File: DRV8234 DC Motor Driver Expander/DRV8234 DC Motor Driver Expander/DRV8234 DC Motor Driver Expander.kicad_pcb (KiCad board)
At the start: 4 copper layers, 73.2 x 31.2 mm, 44 parts, among them IC1 DRV8234RTER, J1 POWER, J2 CNTRL_IN, J3 CNTRL_OUT, J4 I2C, J5 MOTOR

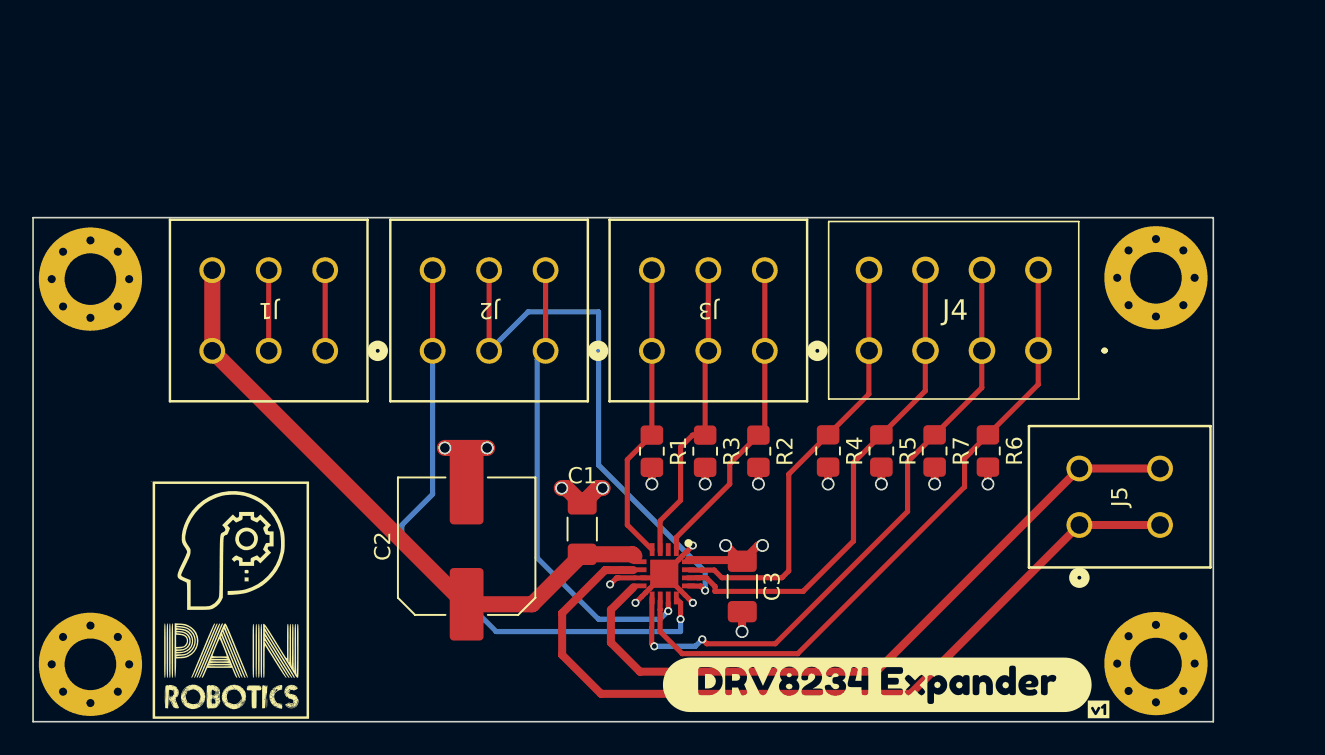
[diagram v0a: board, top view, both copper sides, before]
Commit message: V2
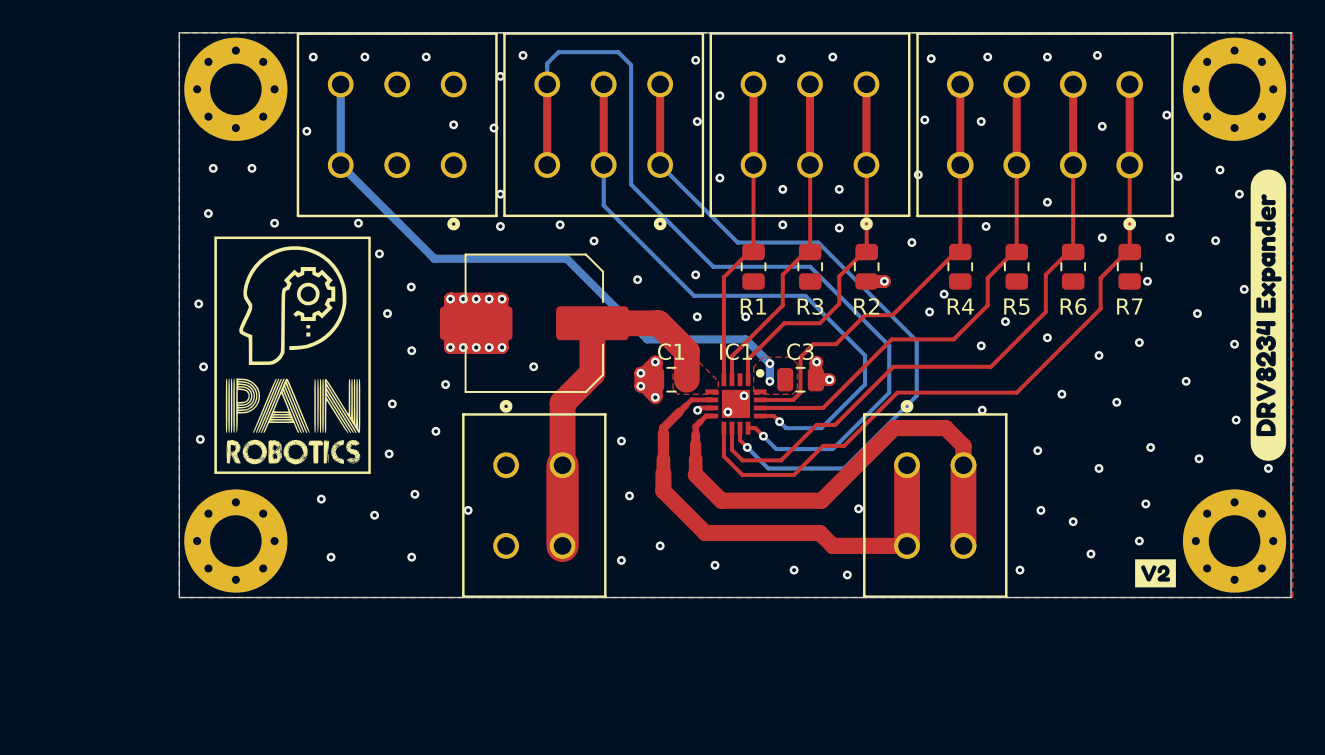
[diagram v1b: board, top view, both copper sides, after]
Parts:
- removed kibuzzard-65A6FC4F: G***, kibuzzard-65A6FC4F
- removed kibuzzard-65A7000E: G***, kibuzzard-65A7000E
- removed kibuzzard-65A7036D: G***, kibuzzard-65A7036D
- removed kibuzzard-65A7039D: G***, kibuzzard-65A7039D
- added J6: CONN_1862055, PCB Footprints:1862055, F.Cu at (110.0, 68.2)
- added kibuzzard-66A118A5: G***, kibuzzard-66A118A5, B.Cu at (113.5, 70.7)
- added kibuzzard-66A118C9: G***, kibuzzard-66A118C9, B.Cu at (122.0, 94.3)
- added kibuzzard-66A1197F: G***, kibuzzard-66A1197F, B.Cu at (120.2, 89.2)
- added kibuzzard-66A11A0B: G***, kibuzzard-66A11A0B, B.Cu at (117.0, 76.0)
- added kibuzzard-66A11A2A: G***, kibuzzard-66A11A2A, B.Cu at (110.0, 75.8)
- added kibuzzard-66A11B65: G***, kibuzzard-66A11B65, F.Cu at (167.5, 82.5)
- added kibuzzard-66A13964: G***, kibuzzard-66A13964, F.Cu at (160.5, 98.5)
- C1, C3: footprint Capacitor_SMD:C_1206_3216Metric_Pad1.33x1.80mm_HandSolder -> Capacitor_SMD:C_0805_2012Metric
- IC1: footprint DRV8234 Footprint:QFN50P300X300X80-17N-D -> PCB Footprints:DRV8234RTER
- J1: value POWER -> CONN_1862042; footprint 1862055 Footprint:CONN_1862055 -> PCB Footprints:1862042
- J2: value CNTRL_IN -> CONN_1862055; footprint 1862055 Footprint:CONN_1862055 -> PCB Footprints:1862055
- J3: value CNTRL_OUT -> CONN_1862055; footprint 1862055 Footprint:CONN_1862055 -> PCB Footprints:1862055
- J4: value I2C -> 1862068; footprint 1862068 Footprint:1862068 -> PCB Footprints:1862068
- J5: value MOTOR -> CONN_1862042; footprint 1862042 Footprint:CONN_1862042 -> PCB Footprints:1862042
- R1, R3: value 10K -> 10k; footprint Resistor_SMD:R_0805_2012Metric_Pad1.20x1.40mm_HandSolder -> Resistor_SMD:R_0805_2012Metric
- R2: value 8.45K -> 1.2k; footprint Resistor_SMD:R_0805_2012Metric_Pad1.20x1.40mm_HandSolder -> Resistor_SMD:R_0805_2012Metric
- R4, R5, R6, R7: value 2.2K -> 2.2k; footprint Resistor_SMD:R_0805_2012Metric_Pad1.20x1.40mm_HandSolder -> Resistor_SMD:R_0805_2012Metric
- moved J1 27.6 mm to (123.8, 96.8), turned to 0 degrees
- moved kibuzzard-65A6FC26 21.8 mm to (123.8, 88.2), turned to 90 degrees
- moved R7 16.6 mm to (158.9, 79.5), turned to 90 degrees
- moved G*** 15.7 mm to (107.0, 85.0)
- moved H1 14.8 mm to (103.5, 68.5)
- moved C2 14.4 mm to (122.0, 83.0), turned to 180 degrees
- moved R5 14.2 mm to (151.9, 79.5), turned to 90 degrees
- moved R4 14.1 mm to (148.4, 79.5), turned to 90 degrees
- moved kibuzzard-65A6FC0C 14.0 mm to (113.5, 75.7)
- moved kibuzzard-65A6FFF9 13.5 mm to (126.3, 70.7), turned to 0 degrees
- moved J2 13.5 mm to (122.8, 68.2)
- moved kibuzzard-65A6FCD9 13.5 mm to (122.8, 75.5)
- moved kibuzzard-65A6FCAC 13.5 mm to (126.3, 75.4)
- moved kibuzzard-65A6FCCE 13.5 mm to (129.8, 76.5), turned to -90 degrees
- moved C3 13.3 mm to (138.5, 86.5), turned to 0 degrees
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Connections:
- C1 pad 1: VCC -> VM
- C2 pad 1: VCC -> VM
- C3 pad 1: +5V -> +3V3
- IC1 pad 16: +5V -> +3V3
- IC1 pad 5: VCC -> VM
- J1 pad 1: +5V -> GND
- J1 pad 2: +5V -> GND
- J1 pad 3: GND -> VM
- J1 pad 4: GND -> VM
- J4 pad 1: A0 -> A1
- J4 pad 2: A0 -> A1
- J4 pad 3: A1 -> A0
- J4 pad 4: A1 -> A0
- R1 pad 1: NFAULT -> VCC_MCU
- R1 pad 2: +5V -> NFAULT
- R3 pad 1: RC_OUT -> VCC_MCU
- R3 pad 2: +5V -> RC_OUT
- R4 pad 1: SCL -> VCC_MCU
- R4 pad 2: +5V -> SCL
- R5 pad 1: SDA -> VCC_MCU
- R5 pad 2: +5V -> SDA
- R6 pad 1: A0 -> VCC_MCU
- R6 pad 2: +5V -> A0
- R7 pad 1: A1 -> VCC_MCU
- R7 pad 2: +5V -> A1
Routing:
- net VCC: track 39.0 -> 0.00 mm
- net +3V3: track 0.00 -> 37.8 mm, vias 0 -> 2
- net GND: track 15.7 -> 42.1 mm, vias 10 -> 96
- net VM: track 0.00 -> 22.9 mm
- net OUT1: track 50.4 -> 29.1 mm
- net +5V: track 17.7 -> 0.00 mm, vias 8 -> 0
- net NSLEEP: track 28.5 -> 43.1 mm
- net IN2: track 38.8 -> 53.3 mm
- net OUT2: track 44.0 -> 30.1 mm
- net A1: track 39.5 -> 44.6 mm, vias 2 -> 0
- net (no net): track 4.67 -> 0.00 mm
- net IN1: track 33.9 -> 37.3 mm
- net IPROPI: track 19.6 -> 22.8 mm
- net RC_OUT: track 19.1 -> 20.5 mm
- net A0: track 41.1 -> 39.9 mm
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- added copper zone on F.Cu, net +3V3
- added copper zone on In2.Cu, net GND
- added copper zone on B.Cu, net VCC_MCU
- added copper zone on F.Cu, net VCC_MCU
- added copper zone on F.Cu, net VM
- removed copper zone on In2.Cu, net +5V
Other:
- board size 73.2 x 31.2 mm -> 68.9 x 35 mm
